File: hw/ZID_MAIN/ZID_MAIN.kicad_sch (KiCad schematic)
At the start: 179 parts, among them J1 Conn 1x04 0.1" Socket, J10 FFC/FPC-40 Socket, J11 JST-PH-K B6B, J12 JST-PH-K B6B, J13 Conn_02x05_PINHDR_2.54mm, J14 USB-C PWR ONLY, J15 Conn 2x03 pin hdr 0.1", J2 JST-PH-K B6B, J3 Conn 1x02 0.1" pin, J4 Conn 1x03 0.1" pin, J5 Conn 1x08 0.1" pin, J6 Conn 1x08 0.1" pin, J7 Conn 2x04 0.1" pin, J8 Conn 2x02 0.1" pin, J9 Conn 2x04 0.1" pin, M1 WS-RP2040-Zero, SW1 SW_Push, SW2 SW_DIP_x02, U1 OSC-20MHz, U10 27WZ06, U11 74LVC125AS, U12 74LVC273, U13 74FCT2245, U14 AS7C1024B, U15 ATF1508AS, U16 74FCT2245, U18 ATF1508AS, U2 74FCT2245, U20 74FCT2244, U22 ATF1504AS-44T, U23 74AHCT00, U24 74FCT2244, U3 24LC32, U4 MIC2775, U5 SST39SF010, U6 74LVC245, U7 74FCT2245, U8 74AHCT14, U9 Z80 C20MHz-PLCC

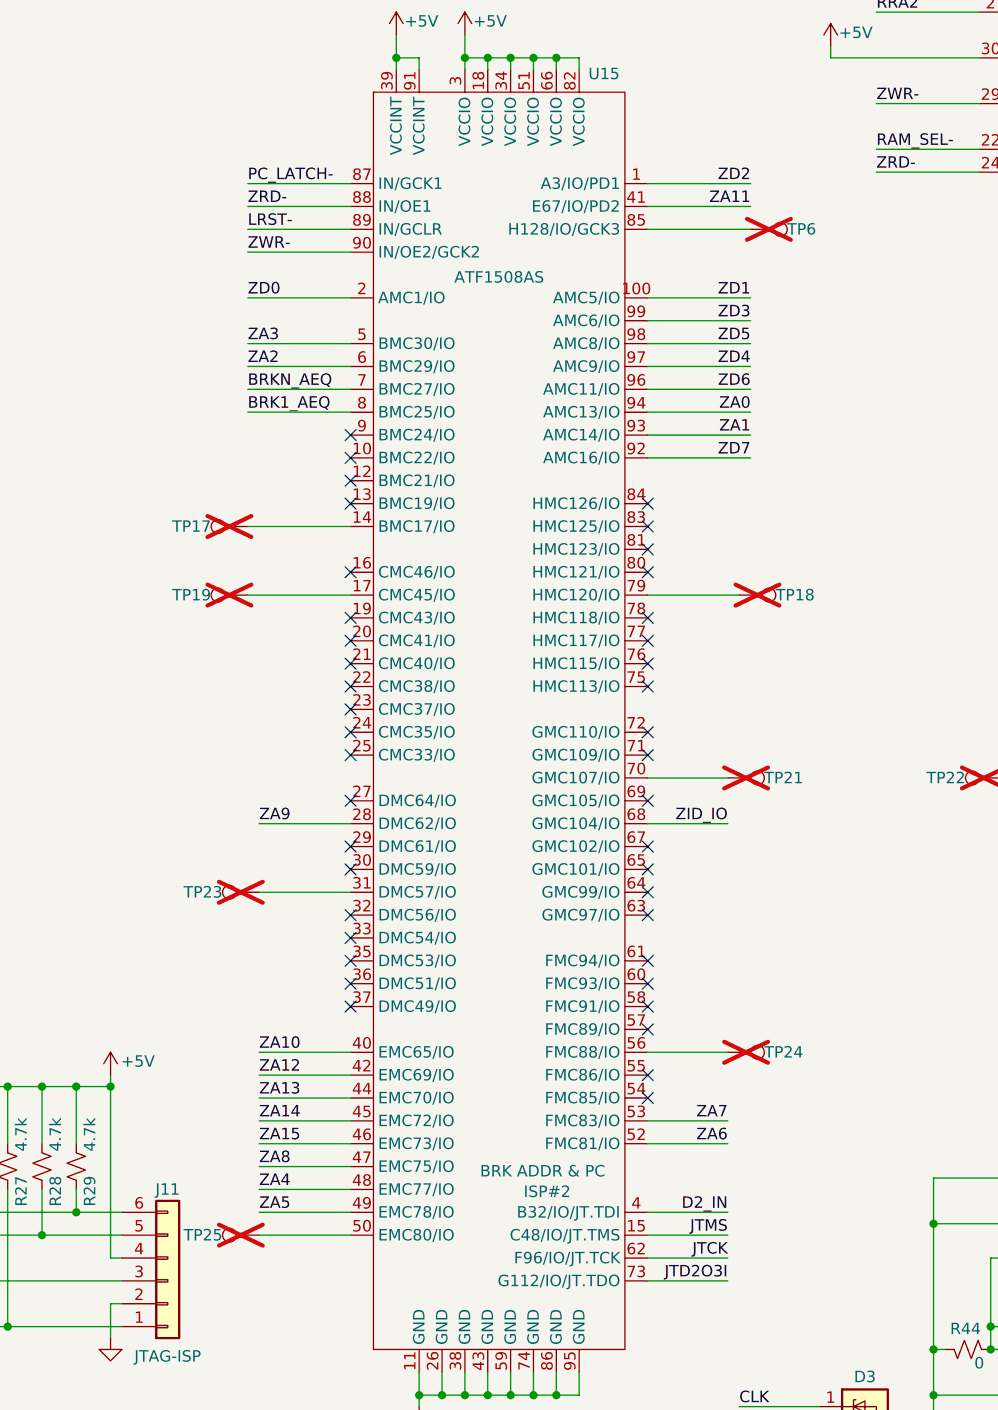
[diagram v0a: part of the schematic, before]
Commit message: PCB: AB+PCL pinout. Exp-BP add position.
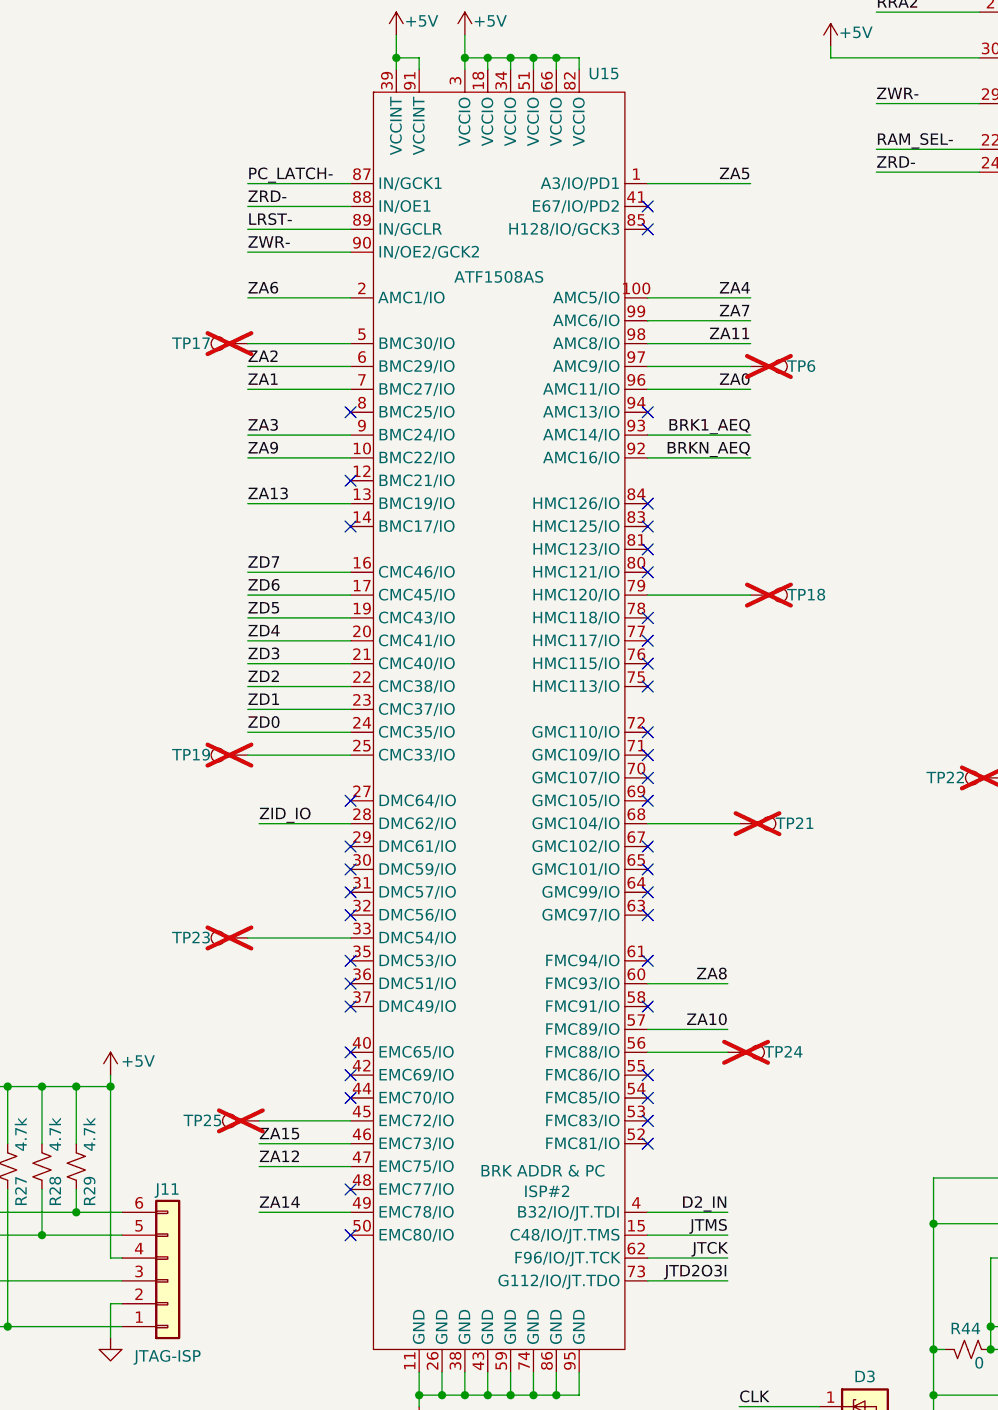
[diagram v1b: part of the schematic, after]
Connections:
- net BRK1_AEQ: now also U15.93 (AMC14/IO); no longer U15.8 (BMC25/IO)
- net BRKN_AEQ: now also U15.92 (AMC16/IO); no longer U15.7 (BMC27/IO)
- net ZA0: now also U15.96 (AMC11/IO); no longer U15.94 (AMC13/IO)
- net ZA1: now also U15.7 (BMC27/IO); no longer U15.93 (AMC14/IO)
- net ZA10: now also U15.57 (FMC89/IO); no longer U15.40 (EMC65/IO)
- net ZA11: now also U15.98 (AMC8/IO); no longer U15.41 (E67/IO/PD2)
- net ZA12: now also U15.47 (EMC75/IO); no longer U15.42 (EMC69/IO)
- net ZA13: now also U15.13 (BMC19/IO); no longer U15.44 (EMC70/IO)
- net ZA14: now also U15.49 (EMC78/IO); no longer U15.45 (EMC72/IO)
- net ZA3: now also U15.9 (BMC24/IO); no longer U15.5 (BMC30/IO)
- net ZA4: now also U15.100 (AMC5/IO); no longer U15.48 (EMC77/IO)
- net ZA5: now also U15.1 (A3/IO/PD1); no longer U15.49 (EMC78/IO)
- net ZA6: now also U15.2 (AMC1/IO); no longer U15.52 (FMC81/IO)
- net ZA7: now also U15.99 (AMC6/IO); no longer U15.53 (FMC83/IO)
- net ZA8: now also U15.60 (FMC93/IO); no longer U15.47 (EMC75/IO)
- net ZA9: now also U15.10 (BMC22/IO); no longer U15.28 (DMC62/IO)
- net ZD0: now also U15.24 (CMC35/IO); no longer U15.2 (AMC1/IO)
- net ZD1: now also U15.23 (CMC37/IO); no longer U15.100 (AMC5/IO)
- net ZD2: now also U15.22 (CMC38/IO); no longer U15.1 (A3/IO/PD1)
- net ZD3: now also U15.21 (CMC40/IO); no longer U15.99 (AMC6/IO)
- net ZD4: now also U15.20 (CMC41/IO); no longer U15.97 (AMC9/IO)
- net ZD5: now also U15.19 (CMC43/IO); no longer U15.98 (AMC8/IO)
- net ZD6: now also U15.17 (CMC45/IO); no longer U15.96 (AMC11/IO)
- net ZD7: now also U15.16 (CMC46/IO); no longer U15.92 (AMC16/IO)
- net ZID_IO: now also U15.28 (DMC62/IO); no longer U15.68 (GMC104/IO)
- net at TP6.1: now also U15.97 (AMC9/IO); no longer U15.85 (H128/IO/GCK3)
- net at TP25.1: now also U15.45 (EMC72/IO); no longer U15.50 (EMC80/IO)
- net at U15.14 (BMC17/IO): no longer TP17.1
- net at TP19.1: now also U15.25 (CMC33/IO); no longer U15.17 (CMC45/IO)
- net at U15.31 (DMC57/IO): no longer TP23.1
- net at U15.33 (DMC54/IO): now also TP23.1
- net at TP21.1: now also U15.68 (GMC104/IO); no longer U15.70 (GMC107/IO)
- new net: TP17.1, U15.5 (BMC30/IO)
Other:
- moved on the sheet: TP17, TP18, TP19, TP21, TP23, TP25, TP6
